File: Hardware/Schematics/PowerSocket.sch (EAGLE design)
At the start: 74 parts, among them T1 BT138-V, T2 BT138-V, T3 BT138-V, T4 BT138-V, T5 BT138-V, T6 BT138-V

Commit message: New board layout
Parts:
- removed ACIN-NULL, ACIN-PHASE, ACOUT-NULL, ACOUT-NULL1, ACOUT-NULL2, ACOUT-PHASE, ACOUT-PHASE1, ACOUT-PHASE2: -, wirepad:3,81/1,4
- removed BUTTON_LED+: BUTTON_VCC, wirepad:2,15/1,0
- removed BUTTON_LED+1, BUTTON_LED+2, BUTTON_LED-, BUTTON_LED-1, BUTTON_LED-2, BUTTON_SWITCH1, BUTTON_SWITCH3, BUTTON_SWITCH5: -, wirepad:2,15/1,0
- removed U$1, U$3, U$4: ACS710, PowerSocket:ACS710
- added AMP1, AMP2, AMP3: ACS710, PowerSocket:ACS710
- added BUTTON1_VCC: (no value), wirepad:2,15/1,0
- added BUTTON2_VCC, BUTTON3_VCC, LED1, LED2, LED3, SWITCH1, SWITCH2, SWITCH3: -, wirepad:2,15/1,0
- added NULL, NULL1-OUT, NULL2-OUT, NULL3-OUT, PHASE, PHASE1-OUT, PHASE2-OUT, PHASE3-OUT: -, wirepad:3,81/1,4
- added R24: 0, eagle-ltspice:RR2010
- R14, R18: device rcl:C-EUC0805 -> rcl:R-EU_R0805
- T1, T2, T3, T4, T5, T6: value BT138-V -> BT138-H; device triac:BT138-V -> triac:BT138-H
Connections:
- net N$25 renamed GATE2
- net N$3 renamed VOLTMETER
- removed net N$15 (its old number): BUTTON_LED-.P, R7.1
- removed net N$2 (its old number): R1.1, RESET.P1, U$2.EN
- removed net N$36 (its old number): ACOUT-PHASE1.P, U$3.IP-, U$3.IP-1, U$3.IP-2, U$3.IP-3
- removed net N$40: U$3.NFAULT
- removed net N$42 (its old number): OK5.C, R16.2
- removed net N$43: OK5.A2, R17.1
- removed net N$45: ACIN-NULL.P, R5.1, T1.A1, T3.A1, T5.A1
- removed net N$46: OK6.C, R18.1
- removed net N$47: OK6.A2, R19.1
- removed net N$49: R19.2, T6.A2, U$4.IP+, U$4.IP+1, U$4.IP+2, U$4.IP+3
- removed net N$50: U$4.NFAULT
- removed net N$51: ACIN-PHASE.P, D1.C, T2.A1, T4.A1, T6.A1
- removed net N$52: R22.2, U$2.IO5
- removed net N$53: R15.2, T4.A2, U$3.IP+, U$3.IP+1, U$3.IP+2, U$3.IP+3
- removed net N$54: R16.1, R18.2, U$2.IO27
- removed net N$55: C9.2, U$1.FILTER
- removed net N$60: C10.2, U$1.VZCR
- removed net N$62: C1.2, U$3.FILTER
- removed net N$63: C4.2, U$3.VZCR
- removed net N$64: C5.2, U$4.FILTER
- removed net N$65: C6.2, U$4.VZCR
- new net AMP1: AMP1.VIOUT, U$2.IO34
- new net AMP2: AMP2.VIOUT, U$2.IO35
- new net AMP3: AMP3.VIOUT, U$2.IO32
- new net BUTTON1: R8.1, SWITCH1.P, U$2.IO22
- new net BUTTON2: R21.1, SWITCH2.P, U$2.IO23
- new net BUTTON3: R23.1, SWITCH3.P, U$2.IO5
- new net GATE1: R3.2, R9.2, U$2.IO25
- new net GATE3: R16.1, R18.1, U$2.IO27
- new net LED1: R7.2, U$2.IO19
- new net LED2: R20.2, U$2.IO18
- new net LED3: R22.2, U$2.IO17
- new net N$24: FLASH.P, FLASH.P1, R2.2, U$2.IO0
- new net N$30: AMP2.VZCR, C4.1
- new net N$66: R1.1, RESET.P, RESET.P1, U$2.EN
- new net NULL: NULL.P, R5.1, T2.A1, T4.A1, T6.A1
- new net PHASE: PHASE.P, R24.2, T1.A1, T3.A1, T5.A1
- new net PHASE1: AMP1.IP+, AMP1.IP+1, AMP1.IP+2, AMP1.IP+3, R10.2, T1.A2
- new net PHASE2: AMP2.IP+, AMP2.IP+1, AMP2.IP+2, AMP2.IP+3, R15.2, T3.A2
- new net PHASE3: AMP3.IP+, AMP3.IP+1, AMP3.IP+2, AMP3.IP+3, R19.2, T5.A2
- net GND: now also AMP1.FAULT_EN, AMP1.GND, AMP2.FAULT_EN, AMP2.GND, AMP3.FAULT_EN, AMP3.GND, C1.2, C10.2, C11.2, C12.2, C13.2, C4.2, C5.2, C6.2, C9.2, FLASH.S, R21.2, R23.2, R8.2, RESET.S1; no longer C1.1, C10.1, C11.1, C12.1, C13.1, C4.1, C5.1, C6.1, C9.1, R21.1, R23.1, R8.1, U$1.FAULT_EN, U$1.GND, U$3.FAULT_EN, U$3.GND, U$4.FAULT_EN, U$4.GND
- net N$1: now also OK1.C, R9.1; no longer ACOUT-NULL.P, R4.2, T1.A2
- net N$10: now also AMP3.IP-, AMP3.IP-1, AMP3.IP-2, AMP3.IP-3, PHASE3-OUT.P; no longer OK2.C, R9.1
- net N$11: now also LED3.P, R22.1; no longer U$2.IO35, U$3.VIOUT
- net N$12: now also AMP1.VZCR, C10.1; no longer U$1.VIOUT, U$2.IO34
- net N$13: now also AMP1.FILTER, C9.1; no longer ACOUT-PHASE.P, U$1.IP-, U$1.IP-1, U$1.IP-2, U$1.IP-3
- net N$14: now also NULL2-OUT.P, T4.A2; no longer ACOUT-NULL1.P, T3.A2
- net N$16: now also OK4.A2, R13.1; no longer BUTTON_LED-1.P, R20.1
- net N$17: now also NULL1-OUT.P, R4.2, T2.A2; no longer BUTTON_SWITCH1.P, R8.2, U$2.IO19
- net N$18: now also OK5.C, R18.2; no longer OK1.A2, R4.1
- net N$20: now also OK1.A2, R10.1; no longer BUTTON_SWITCH3.P, R21.2, U$2.IO18
- net N$21: now also R4.1; no longer R10.1
- net N$23: now also OK3.A2, R15.1; no longer R10.2, T2.A2, U$1.IP+, U$1.IP+1, U$1.IP+2, U$1.IP+3
- net N$26: now also AMP2.IP-, AMP2.IP-1, AMP2.IP-2, AMP2.IP-3, PHASE2-OUT.P; no longer BUTTON_LED-2.P, R22.1
- net N$27: now also AMP1.IP-, AMP1.IP-1, AMP1.IP-2, AMP1.IP-3, PHASE1-OUT.P; no longer U$1.NFAULT
- net N$28: now also R14.1; no longer R12.2
- net N$29: now also OK4.C, R12.2; no longer OK3.A2, R13.1
- net N$31: now also OK6.C, R16.2; no longer R20.2, U$2.IO23
- net N$32: now also AMP2.FILTER, C1.1; no longer OK4.C, R14.1
- net N$33: now also OK6.A2, R17.1; no longer OK4.A2, R15.1
- net N$35: now also OK5.A2, R19.1; no longer ACOUT-PHASE2.P, U$4.IP-, U$4.IP-1, U$4.IP-2, U$4.IP-3
- net N$38: now also AMP3.VZCR, C6.1; no longer ACOUT-NULL2.P, R17.2, T5.A2
- net N$39: now also AMP3.FILTER, C5.1; no longer BUTTON_SWITCH5.P, R23.2, U$2.IO17
- net N$41: now also D1.C, R24.1; no longer U$2.IO32, U$4.VIOUT
- net N$6: now also OK2.C, R3.1; no longer OK1.C, R3.2
- net N$7: now also LED2.P, R20.1; no longer FLASH.P, R2.2, U$2.IO0
- net N$8: now also NULL3-OUT.P, R17.2, T6.A2; no longer R3.1, R9.2, U$2.IO25
- net N$9: now also LED1.P, R7.1; no longer R7.2, U$2.IO22
- net VCC: now also AMP1.VCC, AMP1.VOC, AMP2.VCC, AMP2.VOC, AMP3.VCC, AMP3.VOC, BUTTON1_VCC.P, BUTTON2_VCC.P, BUTTON3_VCC.P, C11.1, C12.1, C13.1; no longer BUTTON_LED+.P, BUTTON_LED+1.P, BUTTON_LED+2.P, C11.2, C12.2, C13.2, U$1.VCC, U$1.VOC, U$3.VCC, U$3.VOC, U$4.VCC, U$4.VOC
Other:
- moved on the sheet: C1, C10, C11, C12, C13, C2, C3, C4, C5, C6, C9, D1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

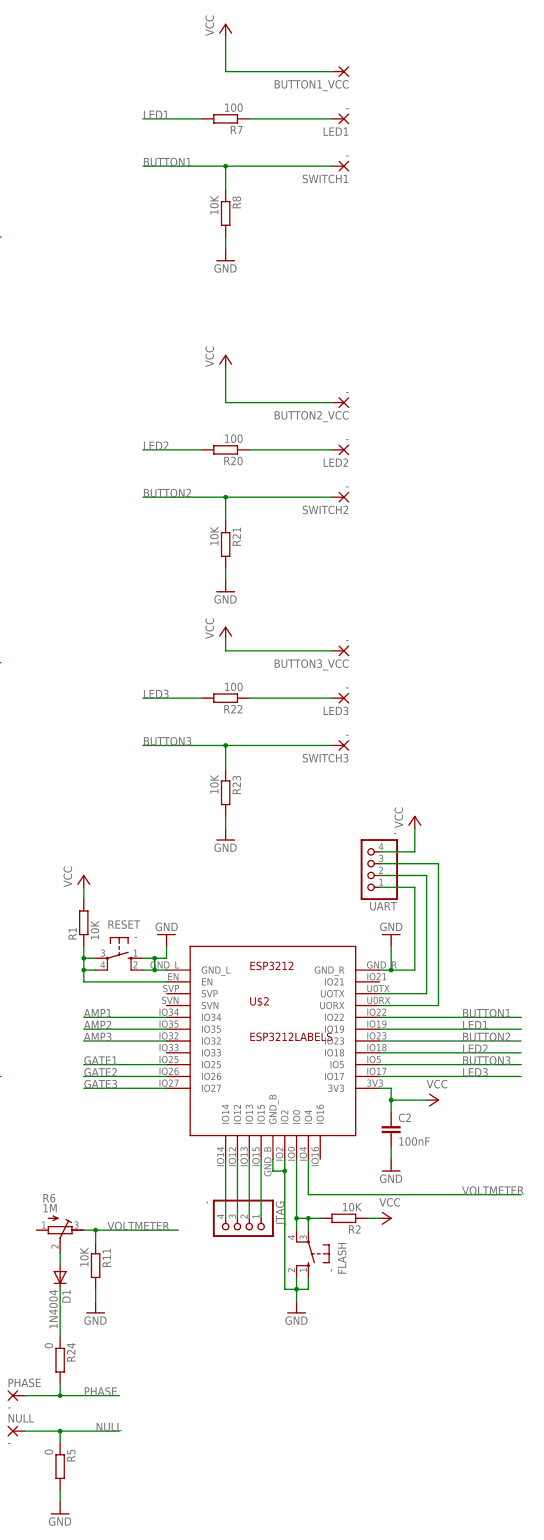
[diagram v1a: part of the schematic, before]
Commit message: Added .brd script.
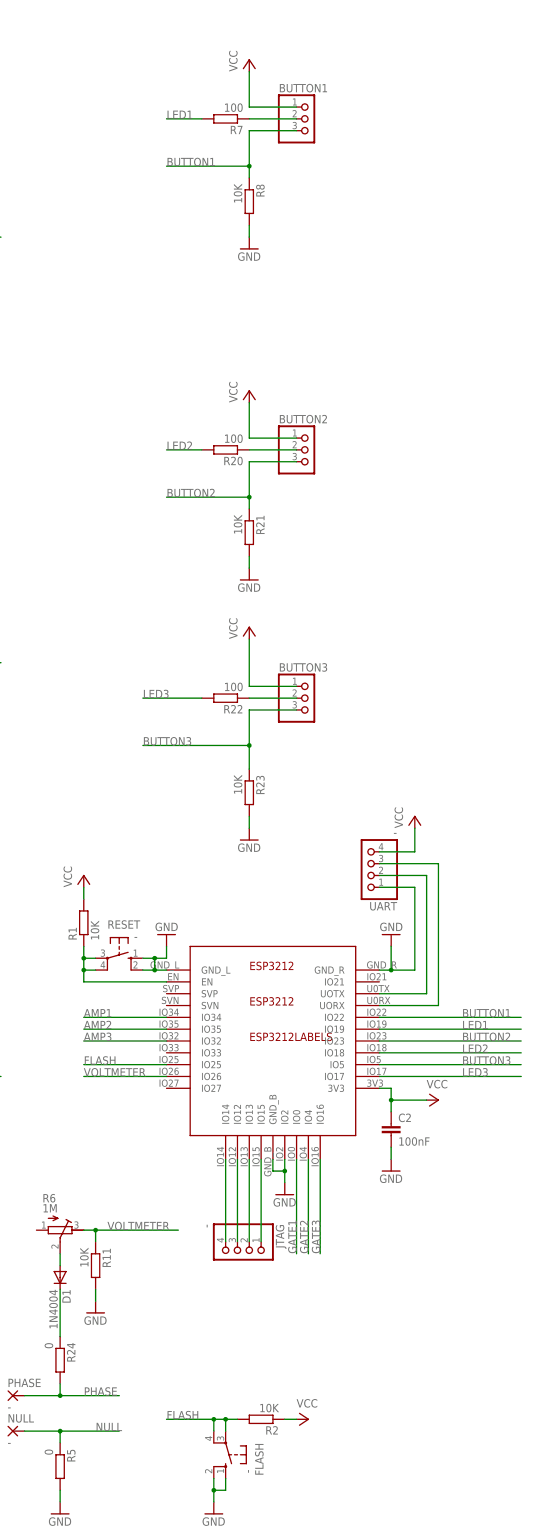
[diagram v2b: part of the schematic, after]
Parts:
- removed BUTTON1_VCC: (no value), wirepad:2,15/1,0
- removed BUTTON2_VCC, BUTTON3_VCC, LED1, LED2, LED3, SWITCH1, SWITCH2, SWITCH3: -, wirepad:2,15/1,0
- added BUTTON1, BUTTON2, BUTTON3: (no value), pinhead:PINHD-1X3
- renumbered U$2 to ESP3212
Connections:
- removed net N$24: ESP3212.IO0, FLASH.P, FLASH.P1, R2.2
- new net FLASH: ESP3212.IO25, FLASH.P, FLASH.P1, R2.2
- net BUTTON1: now also BUTTON1.3; no longer SWITCH1.P
- net BUTTON2: now also BUTTON2.3; no longer SWITCH2.P
- net BUTTON3: now also BUTTON3.3; no longer SWITCH3.P
- net GATE1: now also ESP3212.IO0; no longer ESP3212.IO25
- net GATE2: now also ESP3212.IO4; no longer ESP3212.IO26
- net GATE3: now also ESP3212.IO16; no longer ESP3212.IO27
- net N$11: now also BUTTON3.2; no longer LED3.P
- net N$7: now also BUTTON2.2; no longer LED2.P
- net N$9: now also BUTTON1.2; no longer LED1.P
- net VCC: now also BUTTON1.1, BUTTON2.1, BUTTON3.1; no longer BUTTON1_VCC.P, BUTTON2_VCC.P, BUTTON3_VCC.P
- net VOLTMETER: now also ESP3212.IO26; no longer ESP3212.IO4
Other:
- moved on the sheet: FLASH, JTAG, R2, R21, R23, R8
